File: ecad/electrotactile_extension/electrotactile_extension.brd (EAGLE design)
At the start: 80 x 41.4 mm, 185 parts, among them IC1 DRV8662, J6 1x02 PTH VERT FEMALE, J7 1x02 PTH VERT FEMALE, J8 1x02 PTH VERT FEMALE, J9 1x02 PTH VERT FEMALE, SW1 300mA/4V, SW3 300mA/4V, SW4 300mA/4V

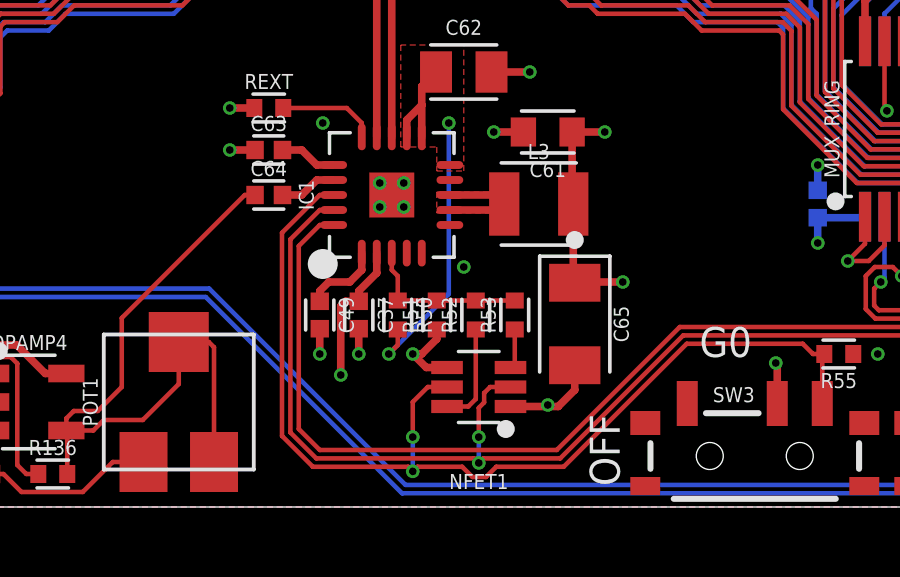
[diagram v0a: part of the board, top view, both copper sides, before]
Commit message: Updates. Meep.
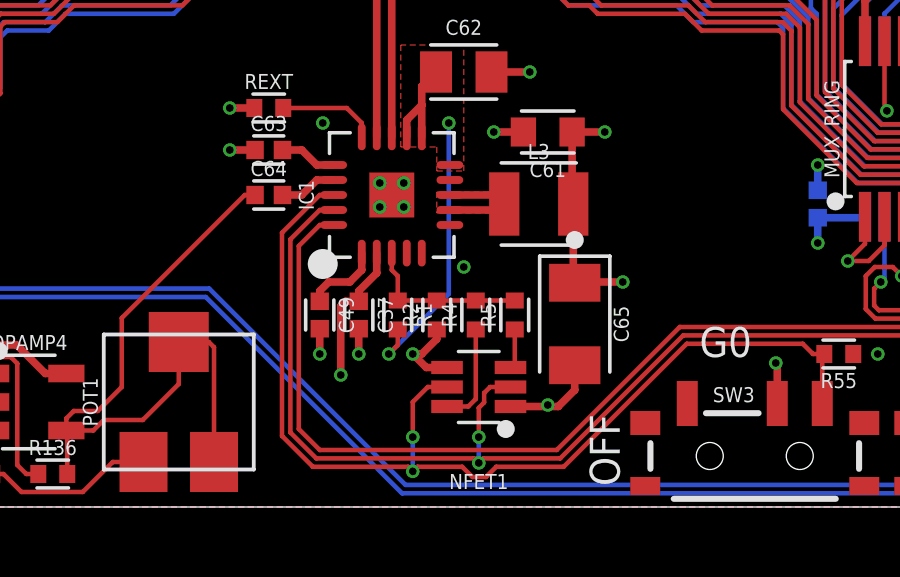
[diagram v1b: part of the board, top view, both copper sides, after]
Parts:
- R2: value 35.7K -> 115K
- R4: value 20K -> 220K
- R5: value 41.2K -> 100K
- renumbered R50 to R1, R51 to R2, R52 to R4, R53 to R5
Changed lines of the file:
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@@
 <?xml version="1.0" encoding="utf-8"?>
 <!DOCTYPE eagle SYSTEM "eagle.dtd">
-<eagle version="9.3.1">
+<eagle version="9.4.0">
 <drawing>
 <settings>
@@
 <grid distance="1" unitdist="mm" unit="mm" style="lines" multiple="1" display="no" altdistance="0.1" altunitdist="mm" altunit="mm"/>
 <layers>
-<layer number="1" name="Top" color="4" fill="1" visible="no" active="yes"/>
-<layer number="2" name="Route2" color="4" fill="6" visible="no" active="yes"/>
+<layer number="1" name="Top" color="4" fill="1" visible="yes" active="yes"/>
+<layer number="2" name="Route2" color="4" fill="6" visible="yes" active="yes"/>
 <layer number="3" name="Route3" color="4" fill="3" visible="no" active="no"/>
 <layer number="4" name="Route4" color="1" fill="4" visible="no" active="no"/>
@@
 <layer number="14" name="Route14" color="1" fill="6" visible="no" active="no"/>
 <layer number="15" name="Route15" color="1" fill="6" visible="yes" active="yes"/>
-<layer number="16" name="Bottom" color="1" fill="1" visible="no" active="yes"/>
+<layer number="16" name="Bottom" color="1" fill="1" visible="yes" active="yes"/>
 <layer number="17" name="Pads" color="2" fill="1" visible="yes" active="yes"/>
 <layer number="18" name="Vias" color="2" fill="1" visible="yes" active="yes"/>
@@
 <attribute name="VALUE" value="0.1uF/50V" x="5.2" y="13.5" size="0.5" layer="27" font="vector" ratio="10" rot="R180" align="top-center"/>
 </element>
-<element name="R50" library="_resistors" package="RESC1005X35_SMD-0402" package3d_urn="urn:adsk.eagle:package:2899165/1" value="768K" x="0.2" y="6.4" smashed="yes" rot="R270">
+<element name="R1" library="_resistors" package="RESC1005X35_SMD-0402" package3d_urn="urn:adsk.eagle:package:2899165/1" value="768K" x="0.2" y="6.4" smashed="yes" rot="R270">
 <attribute name="DATASHEET" value="http://www.yageo.com/documents/recent/PYu-RC_Group_51_RoHS_L_9.pdf" x="14.2" y="26.4" size="1.778" layer="27" rot="R270" display="off"/>
 <attribute name="DIST" value="Digikey" x="14.2" y="26.4" size="1.778" layer="27" rot="R270" display="off"/>
@@
 <attribute name="VALUE" x="-4.1" y="12.665" size="0.25" layer="27" font="vector" ratio="10" align="top-center"/>
 </element>
-<element name="R51" library="_resistors" package="RESC1005X35_SMD-0402" package3d_urn="urn:adsk.eagle:package:2899165/1" value="35.7K" x="1.5" y="6.4" smashed="yes" rot="R90">
+<element name="R2" library="_resistors" package="RESC1005X35_SMD-0402" package3d_urn="urn:adsk.eagle:package:2899165/1" value="115K" x="1.5" y="6.4" smashed="yes" rot="R90">
 <attribute name="DATASHEET" value="http://www.yageo.com/documents/recent/PYu-RC_Group_51_RoHS_L_9.pdf" x="-6.5" y="-24.6" size="1.778" layer="27" rot="R90" display="off"/>
 <attribute name="DIST" value="Digikey" x="-6.5" y="-24.6" size="1.778" layer="27" rot="R90" display="off"/>
@@
 <attribute name="VALUE" x="2.135" y="6.4" size="0.25" layer="27" font="vector" ratio="10" rot="R90" align="top-center"/>
 </element>
-<element name="R52" library="_resistors" package="RESC1005X35_SMD-0402" package3d_urn="urn:adsk.eagle:package:2899165/1" value="20K" x="2.8" y="6.4" smashed="yes" rot="R90">
+<element name="R4" library="_resistors" package="RESC1005X35_SMD-0402" package3d_urn="urn:adsk.eagle:package:2899165/1" value="220K" x="2.8" y="6.4" smashed="yes" rot="R90">
 <attribute name="DATASHEET" value="http://www.yageo.com/documents/recent/PYu-RC_Group_51_RoHS_L_9.pdf" x="-2.2" y="-27.6" size="1.778" layer="27" rot="R90" display="off"/>
 <attribute name="DIST" value="Digikey" x="-2.2" y="-27.6" size="1.778" layer="27" rot="R90" display="off"/>
@@
 <attribute name="VALUE" x="3.435" y="6.4" size="0.25" layer="27" font="vector" ratio="10" rot="R90" align="top-center"/>
 </element>
-<element name="R53" library="_resistors" package="RESC1005X35_SMD-0402" package3d_urn="urn:adsk.eagle:package:2899165/1" value="41.2K" x="4.1" y="6.4" smashed="yes" rot="R90">
+<element name="R5" library="_resistors" package="RESC1005X35_SMD-0402" package3d_urn="urn:adsk.eagle:package:2899165/1" value="100K" x="4.1" y="6.4" smashed="yes" rot="R90">
 <attribute name="DATASHEET" value="http://www.yageo.com/documents/recent/PYu-RC_Group_51_RoHS_L_9.pdf" x="2.1" y="-30.6" size="1.778" layer="27" rot="R90" display="off"/>
 <attribute name="DIST" value="Digikey" x="2.1" y="-30.6" size="1.778" layer="27" rot="R90" display="off"/>
@@
 <contactref element="NFET1" pad="4"/>
 <contactref element="REXT" pad="1"/>
-<contactref element="R51" pad="1"/>
+<contactref element="R2" pad="1"/>
 <contactref element="C65" pad="K"/>
 <contactref element="R54" pad="1"/>
@@
 <contactref element="IC1" pad="11"/>
 <contactref element="IC1" pad="12"/>
-<contactref element="R50" pad="2"/>
+<contactref element="R1" pad="2"/>
 <contactref element="C62" pad="1"/>
 <wire x1="1" y1="12.3373" x2="1" y2="13.4" width="0.254" layer="1"/>
@@
 </signal>
 <signal name="FB">
-<contactref element="R50" pad="1"/>
+<contactref element="R1" pad="1"/>
 <contactref element="IC1" pad="3"/>
-<contactref element="R52" pad="2"/>
-<contactref element="R53" pad="2"/>
-<contactref element="R51" pad="2"/>
+<contactref element="R4" pad="2"/>
+<contactref element="R5" pad="2"/>
+<contactref element="R2" pad="2"/>
 <wire x1="0" y1="8.4627" x2="0" y2="7.9" width="0.1524" layer="1"/>
 <wire x1="0.2" y1="7.7" x2="0.2" y2="6.8825" width="0.1524" layer="1"/>
@@
 <signal name="N$49">
 <contactref element="NFET1" pad="6"/>
-<contactref element="R52" pad="1"/>
+<contactref element="R4" pad="1"/>
 <wire x1="1.8427" y1="3.35" x2="2.55" y2="3.35" width="0.1524" layer="1"/>
 <wire x1="2.8" y1="5.9175" x2="2.8" y2="3.6" width="0.1524" layer="1"/>
@@
 <signal name="N$51">
 <contactref element="NFET1" pad="3"/>
-<contactref element="R53" pad="1"/>
+<contactref element="R5" pad="1"/>
 <wire x1="4.1" y1="5.9175" x2="4.1" y2="4.7927" width="0.1524" layer="1"/>
 <wire x1="3.9573" y1="4.65" x2="4.1" y2="4.7927" width="0.1524" layer="1"/>
